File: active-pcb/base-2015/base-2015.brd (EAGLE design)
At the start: 50.5 x 64.8 mm, 5 parts, among them X1 MINI-USB-32005-201

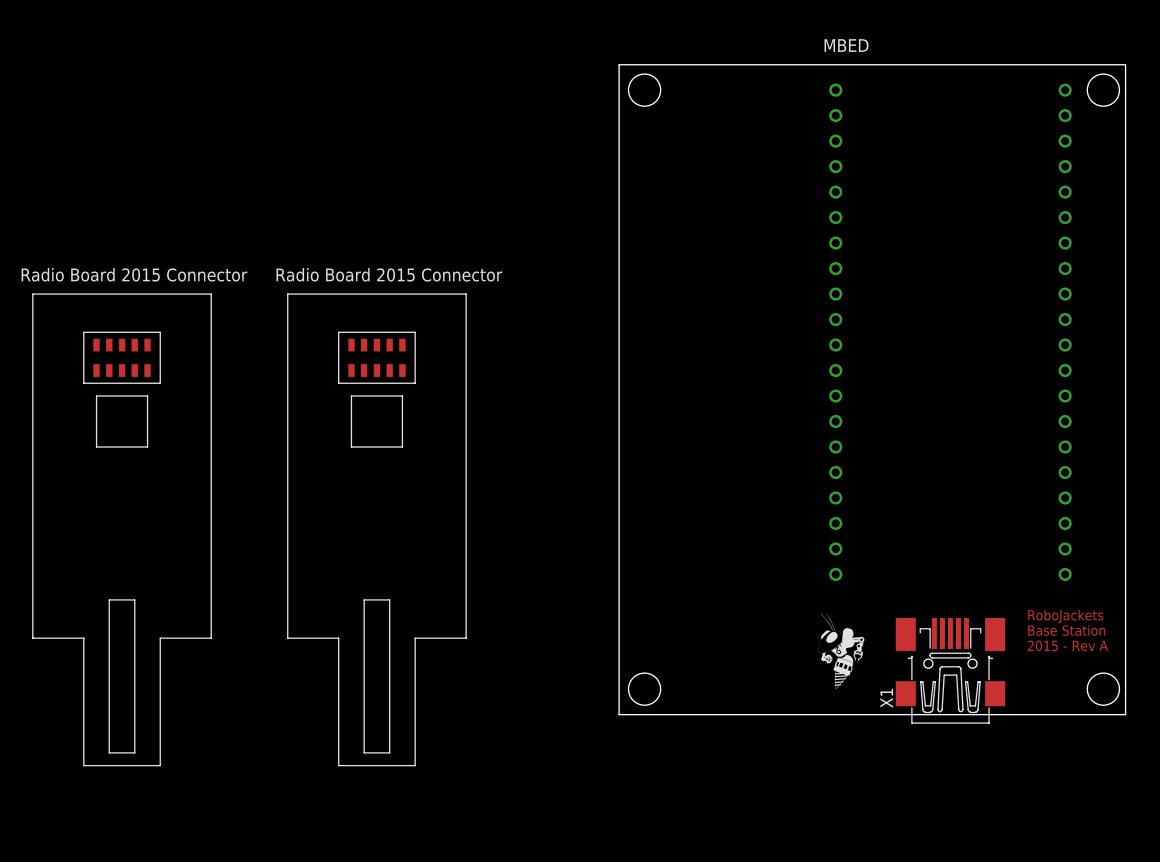
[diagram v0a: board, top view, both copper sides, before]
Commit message: re-arranged board
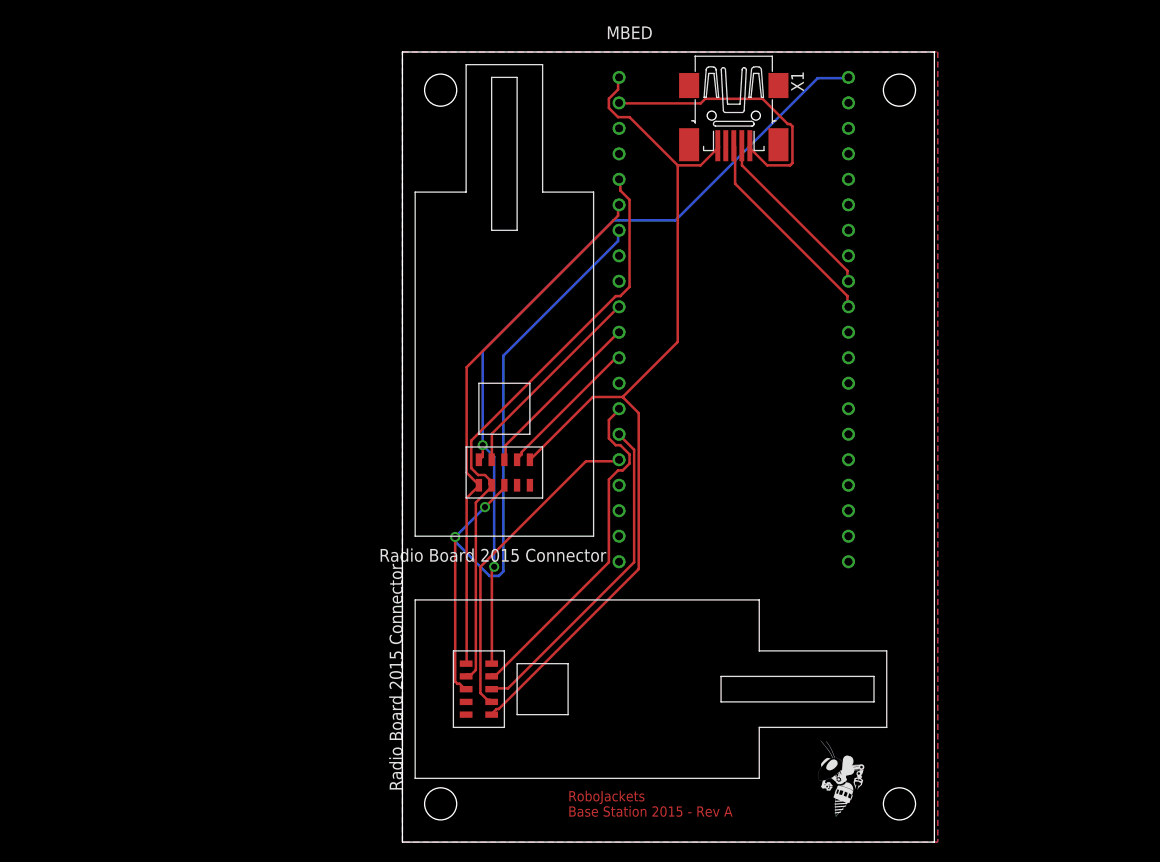
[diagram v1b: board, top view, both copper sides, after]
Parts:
- moved X1 58.7 mm to (33.0, 72.4), turned to 270 degrees
- moved U$2 52.1 mm to (6.35, 12.7), turned to 90 degrees
- moved U$1 22.6 mm to (12.7, 35.6), turned to 180 degrees
- moved MBED 21.6 mm to (33.0, 52.1)
- moved U$3 12.7 mm to (43.2, 2.54)
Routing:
- net N$16: track 0.00 -> 93.4 mm
- net N$8: track 0.00 -> 81.1 mm, vias 0 -> 2
- net N$17: track 0.00 -> 68.7 mm, vias 0 -> 2
- net N$2: track 0.00 -> 59.4 mm
- net N$3: track 0.00 -> 53.0 mm
- net N$14: track 0.00 -> 34.4 mm
- net N$4: track 0.00 -> 32.8 mm
- net N$13: track 0.00 -> 32.3 mm
- net N$5: track 0.00 -> 27.6 mm
- net N$7: track 0.00 -> 20.8 mm
- net N$12: track 0.00 -> 20.5 mm
- net N$6: track 0.00 -> 17.9 mm
- net N$10: track 0.00 -> 17.5 mm
- net N$9: track 0.00 -> 14.8 mm
- added copper zone on layer 1, net GND
- added copper zone on layer 16, net GND
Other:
- board size 50.5 x 64.8 mm -> 53 x 78.7 mm
